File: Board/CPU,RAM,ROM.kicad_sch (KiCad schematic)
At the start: 17 parts, among them IC1 74LVC125, IC6 741G04DBV, IC7 74LVC138, U1 IS61WV51216EDALL, X3 SG-8002CE

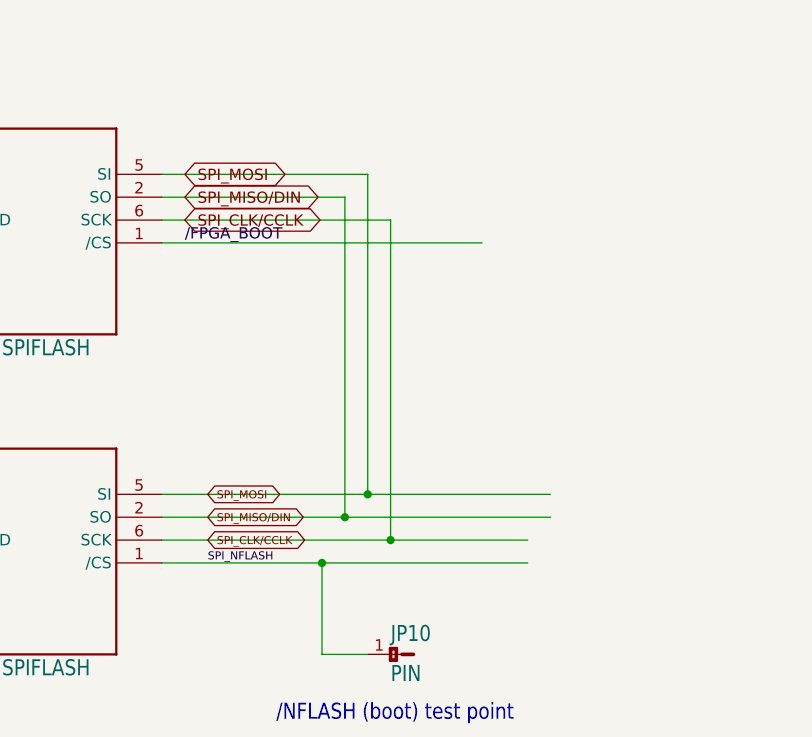
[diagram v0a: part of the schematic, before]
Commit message: layout work
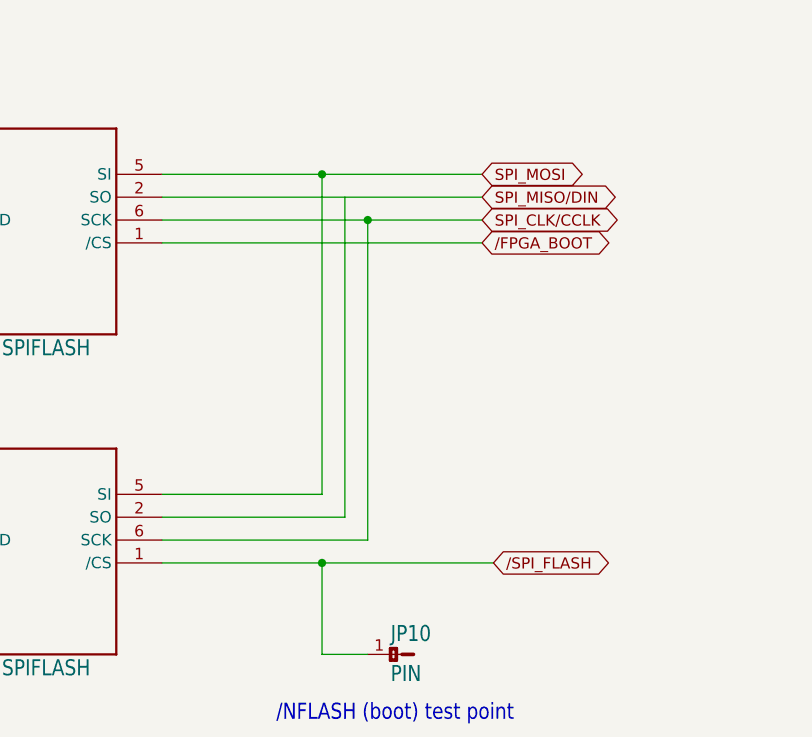
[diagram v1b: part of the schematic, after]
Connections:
- net SPI_MISO/DIN: no longer U$4.2 (SO)
- net /FPGA_BOOT renamed /FPGA_BOOT
- net SPI_NFLASH renamed /SPI_FLASH
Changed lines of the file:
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@@
 	)
 	(junction
+		(at 90.17 83.82)
+		(diameter 0)
+		(color 0 0 0 0)
+	)
+	(junction
 		(at 224.79 184.15)
 		(diameter 0)
@@
 	)
 	(junction
+		(at 90.17 40.64)
+		(diameter 0)
+		(color 0 0 0 0)
+	)
+	(junction
 		(at 181.61 207.01)
 		(diameter 0)
@@
 	)
 	(junction
+		(at 95.25 45.72)
+		(diameter 0)
+		(color 0 0 0 0)
+	)
+	(junction
 		(at 52.705 212.09)
 		(diameter 0)
@@
 	)
 	(junction
-		(at 95.25 76.2)
-		(diameter 0)
-		(color 0 0 0 0)
-	)
-	(junction
 		(at 353.06 74.93)
 		(diameter 0)
@@
 	)
 	(junction
-		(at 97.79 81.28)
-		(diameter 0)
-		(color 0 0 0 0)
-	)
-	(junction
 		(at 256.54 72.39)
 		(diameter 0)
@@
 	)
 	(junction
-		(at 90.17 83.82)
-		(diameter 0)
-		(color 0 0 0 0)
-	)
-	(junction
 		(at 229.87 148.59)
 		(diameter 0)
@@
 		(color 0 0 0 0)
 	)
-	(junction
-		(at 92.71 78.74)
-		(diameter 0)
-		(color 0 0 0 0)
-	)
 	(wire
 		(pts
@@
 	(wire
 		(pts
-			(xy 72.39 81.28) (xy 97.79 81.28)
+			(xy 72.39 81.28) (xy 95.25 81.28)
 		)
 		(stroke
@@
 	(wire
 		(pts
+			(xy 95.25 45.72) (xy 107.95 45.72)
+		)
+		(stroke
+			(width 0.1524)
+			(type solid)
+		)
+	)
+	(wire
+		(pts
 			(xy 214.63 163.83) (xy 224.79 163.83)
 		)
@@
 	(wire
 		(pts
-			(xy 72.39 43.18) (xy 92.71 43.18)
+			(xy 72.39 43.18) (xy 107.95 43.18)
 		)
 		(stroke
@@
 	(wire
 		(pts
-			(xy 72.39 76.2) (xy 95.25 76.2)
+			(xy 72.39 76.2) (xy 90.17 76.2)
 		)
 		(stroke
@@
 	(wire
 		(pts
-			(xy 92.71 78.74) (xy 115.57 78.74)
-		)
-		(stroke
-			(width 0.1524)
-			(type solid)
-		)
-	)
-	(wire
-		(pts
 			(xy 46.99 181.61) (xy 55.88 181.61)
 		)
@@
 	(wire
 		(pts
-			(xy 97.79 81.28) (xy 97.79 45.72)
+			(xy 95.25 81.28) (xy 95.25 45.72)
 		)
 		(stroke
@@
 	(wire
 		(pts
-			(xy 72.39 40.64) (xy 95.25 40.64)
+			(xy 72.39 40.64) (xy 90.17 40.64)
 		)
 		(stroke
@@
 	(wire
 		(pts
+			(xy 90.17 40.64) (xy 107.95 40.64)
+		)
+		(stroke
+			(width 0.1524)
+			(type solid)
+		)
+	)
+	(wire
+		(pts
 			(xy 232.41 194.31) (xy 217.17 194.31)
 		)
@@
 	(wire
 		(pts
-			(xy 95.25 40.64) (xy 95.25 76.2)
+			(xy 90.17 40.64) (xy 90.17 76.2)
 		)
 		(stroke
@@
 	(wire
 		(pts
-			(xy 97.79 81.28) (xy 113.03 81.28)
-		)
-		(stroke
-			(width 0.1524)
-			(type solid)
-		)
-	)
-	(wire
-		(pts
 			(xy 86.36 173.99) (xy 92.71 173.99)
 		)
@@
 	(wire
 		(pts
-			(xy 72.39 45.72) (xy 97.79 45.72)
+			(xy 72.39 45.72) (xy 95.25 45.72)
 		)
 		(stroke
@@
 	(wire
 		(pts
-			(xy 90.17 83.82) (xy 113.03 83.82)
+			(xy 90.17 83.82) (xy 109.22 83.82)
 		)
 		(stroke
@@
 	(wire
 		(pts
-			(xy 95.25 76.2) (xy 115.57 76.2)
-		)
-		(stroke
-			(width 0.1524)
-			(type solid)
-		)
-	)
-	(wire
-		(pts
 			(xy 86.36 171.45) (xy 93.98 171.45)
 		)
@@
 		)
 	)
-	(label "SPI_NFLASH"
-		(at 77.47 83.82 0)
-		(effects
-			(font
-				(size 0.889 0.889)
-			)
-			(justify left bottom)
-		)
-	)
 	(label "VPB"
 		(at 219.71 148.59 0)
@@
 		)
 	)
-	(label "/FPGA_BOOT"
-		(at 74.93 48.26 0)
-		(effects
-			(font
-				(size 1.2446 1.2446)
-			)
-			(justify left bottom)
-		)
-	)
 	(global_label "A8"
 		(shape input)
@@
 		)
 	)
+	(global_label "{slash}FPGA_BOOT"
+		(shape bidirectional)
+		(at 107.95 48.26 0)
+		(fields_autoplaced yes)
+		(effects
+			(font
+				(size 1.2446 1.2446)
+			)
+			(justify left)
+		)
+		(property "Intersheetrefs" "${INTERSHEET_REFS}"
+			(at 123.6399 48.26 0)
+			(hide yes)
+			(show_name no)
+			(do_not_autoplace no)
+			(effects
+				(font
+					(size 1.27 1.27)
+				)
+				(justify left)
+			)
+		)
+	)
 	(global_label "SPI_MOSI"
 		(shape bidirectional)
-		(at 74.93 40.64 0)
+		(at 107.95 40.64 0)
 		(fields_autoplaced yes)
 		(effects
@@
 		)
 		(property "Intersheetrefs" "${INTERSHEET_REFS}"
-			(at 87.4194 40.64 0)
+			(at 120.4394 40.64 0)
 			(hide yes)
 			(show_name no)
@@
 	(global_label "SPI_MISO/DIN"
 		(shape bidirectional)
-		(at 74.93 43.18 0)
+		(at 107.95 43.18 0)
 		(fields_autoplaced yes)
 		(effects
@@
 		)
 		(property "Intersheetrefs" "${INTERSHEET_REFS}"
-			(at 91.8645 43.18 0)
+			(at 124.8845 43.18 0)
 			(hide yes)
 			(show_name no)
@@
 	(global_label "SPI_CLK/CCLK"
 		(shape bidirectional)
-		(at 74.93 45.72 0)
+		(at 107.95 45.72 0)
 		(fields_autoplaced yes)
 		(effects
@@
 		)
 		(property "Intersheetrefs" "${INTERSHEET_REFS}"
-			(at 92.457 45.72 0)
+			(at 125.477 45.72 0)
 			(hide yes)
 			(show_name no)
@@
 		)
 	)
-	(global_label "SPI_CLK/CCLK"
-		(shape bidirectional)
-		(at 77.47 81.28 0)
-		(fields_autoplaced yes)
-		(effects
-			(font
-				(size 0.889 0.889)
-			)
-			(justify left)
-		)
-		(property "Intersheetrefs" "${INTERSHEET_REFS}"
-			(at 89.9894 81.28 0)
-			(hide yes)
-			(show_name no)
-			(do_not_autoplace no)
-			(effects
-				(font
-					(size 1.27 1.27)
-				)
-				(justify left)
-			)
-		)
-	)
 	(global_label "/NMI"
 		(shape bidirectional)
@@
 		)
 	)
-	(global_label "SPI_MOSI"
-		(shape bidirectional)
-		(at 77.47 76.2 0)
-		(fields_autoplaced yes)
-		(effects
-			(font
-				(size 0.889 0.889)
-			)
-			(justify left)
-		)
-		(property "Intersheetrefs" "${INTERSHEET_REFS}"
-			(at 86.391 76.2 0)
-			(hide yes)
-			(show_name no)
-			(do_not_autoplace no)
-			(effects
-				(font
-					(size 1.27 1.27)
-				)
-				(justify left)
-			)
-		)
-	)
 	(global_label "/IRQ"
 		(shape bidirectional)
@@
 		)
 	)
+	(global_label "{slash}SPI_FLASH"
+		(shape bidirectional)
+		(at 109.22 83.82 0)
+		(fields_autoplaced yes)
+		(effects
+			(font
+				(size 1.2446 1.2446)
+			)
+			(justify left)
+		)
+		(property "Intersheetrefs" "${INTERSHEET_REFS}"
+			(at 124.1393 83.82 0)
+			(hide yes)
+			(show_name no)
+			(do_not_autoplace no)
+			(effects
+				(font
+					(size 1.27 1.27)
+				)
+				(justify left)
+			)
+		)
+	)
 	(global_label "D7"
 		(shape bidirectional)
@@
 			(hide yes)
 			(show_name no)
-			(do_not_autoplace no)
-			(effects
-				(font
-					(size 1.27 1.27)
-				)
-				(justify left)
-			)
-		)
-	)
-	(global_label "SPI_MISO/DIN"
-		(shape bidirectional)
-		(at 77.47 78.74 0)
-		(fields_autoplaced yes)
-		(effects
-			(font
-				(size 0.889 0.889)
-			)
-			(justify left)
-		)
-		(property "Intersheetrefs" "${INTERSHEET_REFS}"
-			(at 89.5659 78.74 0)
-			(hide yes)
-			(show_name no)
